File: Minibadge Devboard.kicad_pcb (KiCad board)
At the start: 2 copper layers, 30.5 x 48.3 mm, 45 parts, among them J1 External power, J2 External switch, SW1 Power, SW3 SPEED, SW4 NTC

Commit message: Update values
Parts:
- C11: value C_SS -> 0.1uF
- CHARGE: value RED -> CHARGE
- PWR: value RED -> PWR
- R9: value R_ILIM -> 30kΩ
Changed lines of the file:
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@@
 			)
 		)
-		(property "LCSC Part #" ""
+		(property "LCSC Part #" "C8218"
 			(at 0 0 180)
 			(unlocked yes)
@@
 			)
 		)
-		(property "Value" "C_SS"
+		(property "Value" "0.1uF"
 			(at 0 1.43 0)
 			(layer "F.Fab")
@@
 			)
 		)
-		(property "LCSC Part #" ""
+		(property "LCSC Part #" "C14663"
 			(at 0 0 0)
 			(unlocked yes)
@@
 			)
 		)
-		(property "Value" "R_ILIM"
+		(property "Value" "30kΩ"
 			(at 0 1.43 0)
 			(layer "F.Fab")
@@
 			)
 		)
-		(property "LCSC Part #" ""
+		(property "LCSC Part #" "C22984"
 			(at 0 0 0)
 			(unlocked yes)
@@
 			)
 		)
-		(property "Value" "RED"
+		(property "Value" "CHARGE"
 			(at 0 1.43 0)
 			(layer "F.Fab")
@@
 			)
 		)
-		(property "LCSC Part #" ""
+		(property "LCSC Part #" "C8218"
 			(at 0 0 0)
 			(unlocked yes)
@@
 			)
 		)
-		(property "Value" "RED"
+		(property "Value" "PWR"
 			(at 0 1.43 0)
 			(layer "F.Fab")

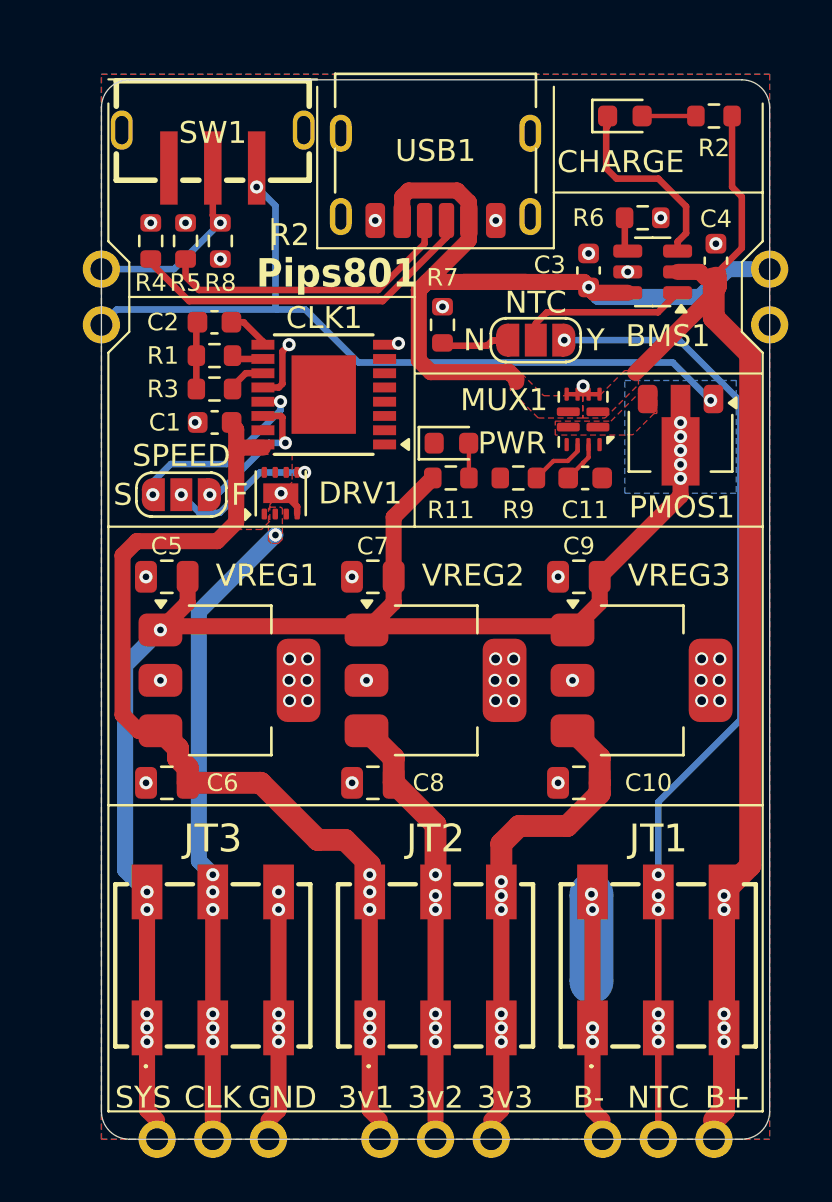
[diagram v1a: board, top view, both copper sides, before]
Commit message: Update Minibadge Devboard.kicad_pcb
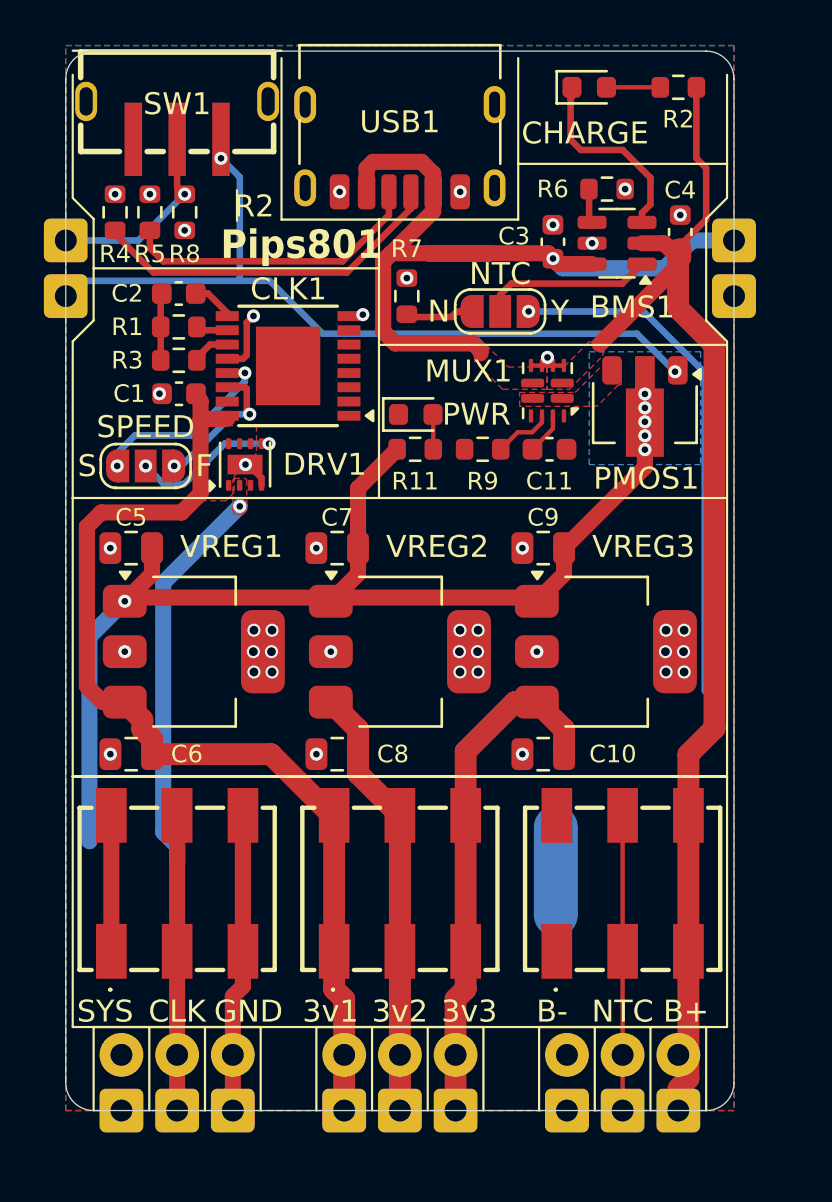
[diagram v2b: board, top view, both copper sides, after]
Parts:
- added ?: , , F.Cu at (104.1, 81.3)
- added ?: , , F.Cu at (94.0, 81.3)
- added ?: , , F.Cu at (114.3, 81.3)
- added ?: , , F.Cu at (101.6, 81.3)
- added ?: , , F.Cu at (96.5, 81.3)
- added ?: , , F.Cu at (106.7, 81.3)
- added ?: , , F.Cu at (111.8, 81.3)
- added ?: , , F.Cu at (91.4, 81.3)
- added ?: , , F.Cu at (116.8, 81.3)
- moved JT1 3.85 mm to (114.3, 73.7)
- moved JT2 3.85 mm to (104.1, 73.7)
- moved JT3 3.85 mm to (94.0, 73.7)
- moved NT1 3.46 mm to (111.3, 72.9)
- moved C10 2.09 mm to (110.7, 67.6)
- moved C8 2.09 mm to (101.3, 67.6)
- moved JC1 2.09 mm to (114.3, 83.8)
- moved JC2 2.09 mm to (104.1, 83.8)
- moved C1 2.09 mm to (94.1, 51.1)
- moved C11 2.09 mm to (111.0, 53.7)
- moved C4 2.09 mm to (116.9, 43.7)
- moved C7 2.09 mm to (101.3, 58.2)
- moved C9 2.09 mm to (110.7, 58.2)
- moved CHARGE 2.09 mm to (112.8, 37.1)
- moved CLK1 2.09 mm to (99.0, 49.9)
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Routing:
- net -BATT: track 10.5 -> 0.00 mm, vias 4 -> 0
- net NTC: track 45.4 -> 36.6 mm, vias 7 -> 1
- net SYS: track 66.3 -> 60.5 mm, vias 11 -> 6
- net CLK: track 28.4 -> 30.6 mm, vias 7 -> 1
- net GND: track 16.8 -> 19.0 mm, vias 47 -> 42
- net +3.3V-3: track 21.6 -> 22.6 mm, vias 6 -> 0
- net +3.3V-1: track 45.6 -> 46.0 mm, vias 6 -> 0
- net +BATT: track 54.7 -> 54.5 mm, vias 5 -> 0
- net +3.3V-2: track 19.1 -> 18.9 mm, vias 6 -> 0
